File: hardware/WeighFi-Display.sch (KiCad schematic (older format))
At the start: 43 parts, among them P1 CONN_12, P10 CONN_4, P11 CONN_1, P12 CONN_1, P13 CONN_1, P14 CONN_1, P15 CONN_1, P16 CONN_1, P17 CONN_1, P18 CONN_1, P19 CONN_1, P2 CONN_1, P20 CONN_1, P21 CONN_1, P22 CONN_1, P23 CONN_1, P24 CONN_1, P25 CONN_1, P26 CONN_1, P27 CONN_13, P3 CONN_1, P4 CONN_1, P5 CONN_1, P6 CONN_1, P7 CONN_1, P8 CONN_1, P9 CONN_1, U1 ADS1131, U2 PCF8566

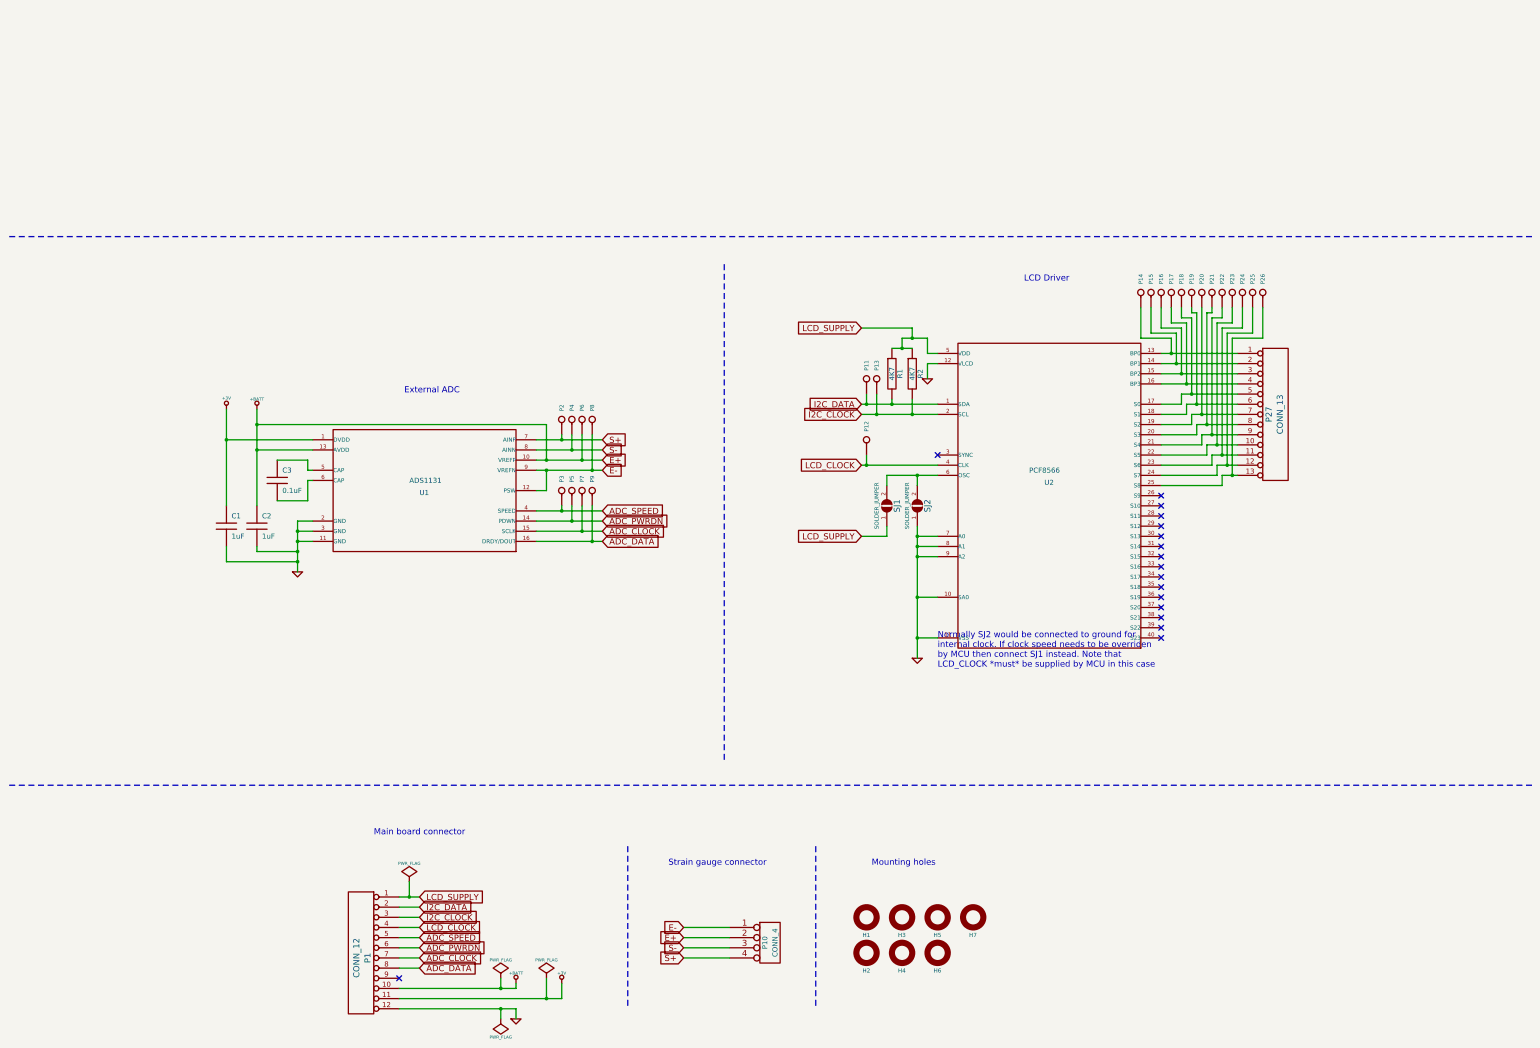
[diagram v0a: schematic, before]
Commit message: Refine schematics, generate new netlists
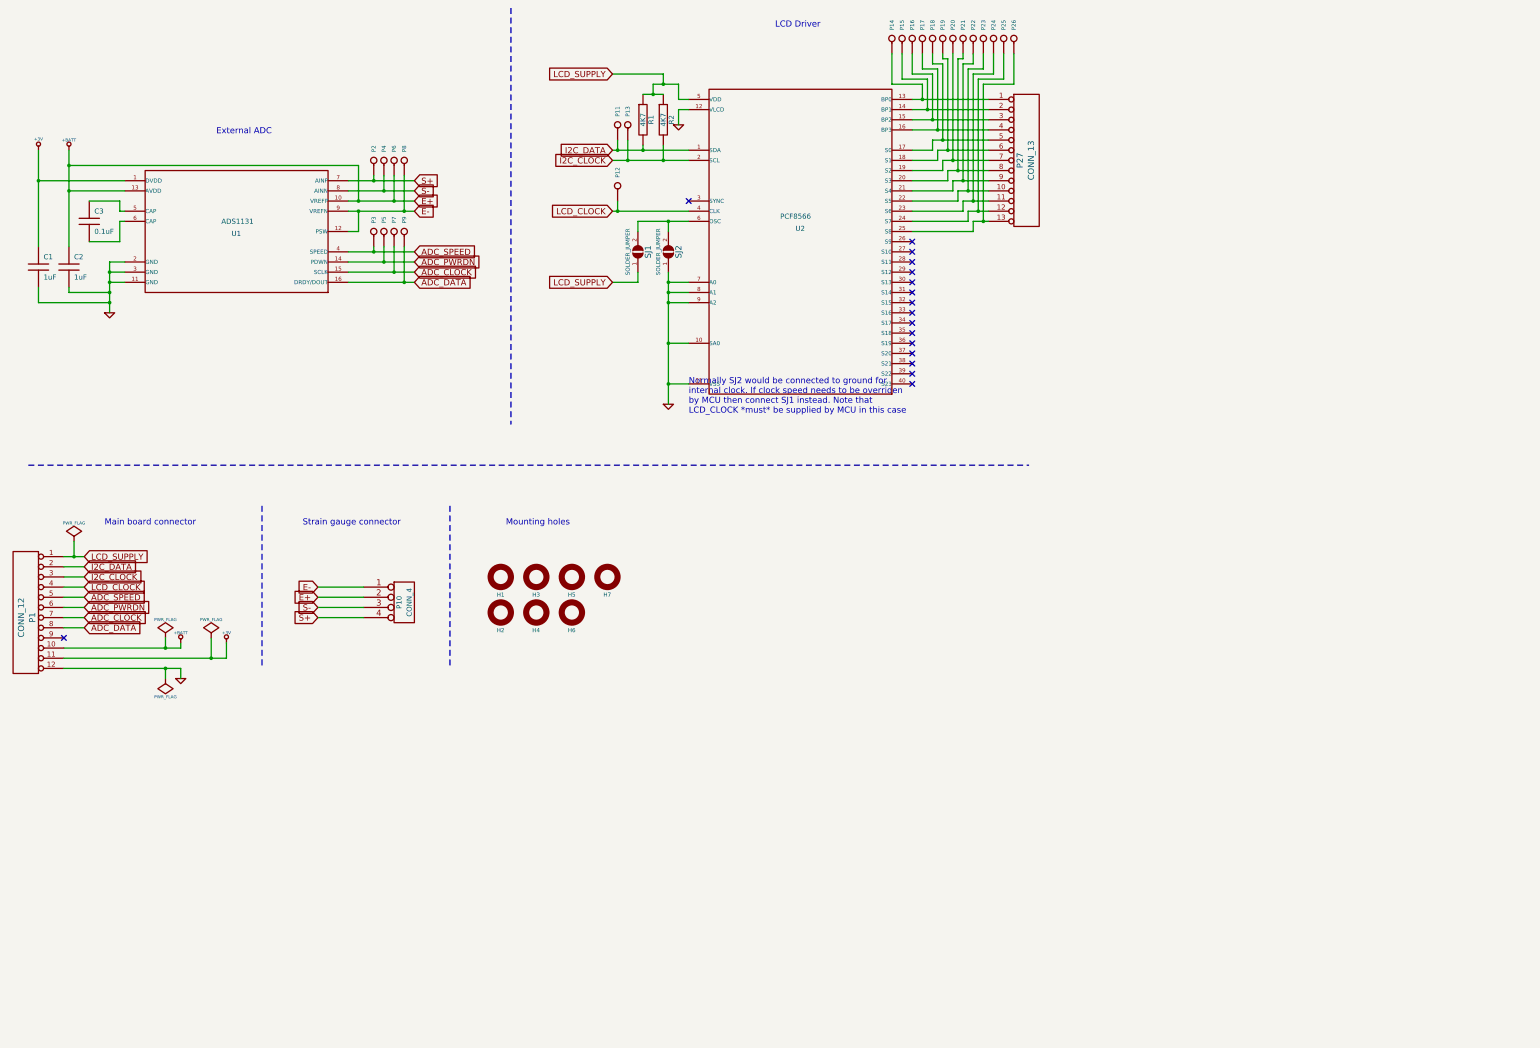
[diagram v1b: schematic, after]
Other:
- moved on the sheet: C1, C2, C3, H1, H2, H3, H4, H5, H6, H7, P1, P10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
